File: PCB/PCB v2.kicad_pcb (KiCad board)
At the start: 4 copper layers, 55.3 x 42.7 mm, 91 parts, among them J1 Conn_01x02_Pin, J3 6871XX182122_687110182122, J5 Conn_01x03_Pin, J7 Conn_01x07_Pin, U1 LT3483AxS6, U11 OPA4350EA_250, U12 OPA4350EA_250, U13 OPA4350EA_250, U2 LT1761-2.5, U3 LT1964-BYP, U5 AD7606, U6 OPA4350EA_250

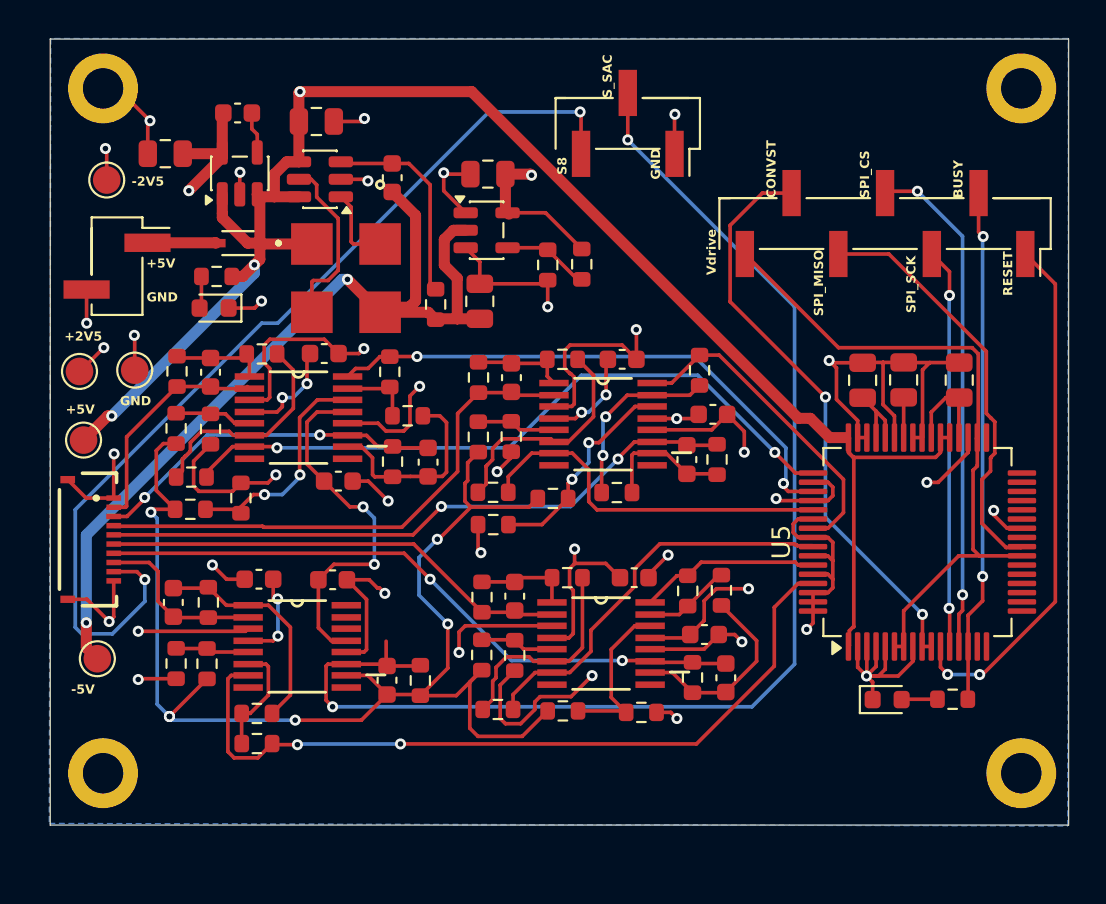
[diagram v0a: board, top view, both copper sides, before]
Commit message: Modifiche accordate fatte
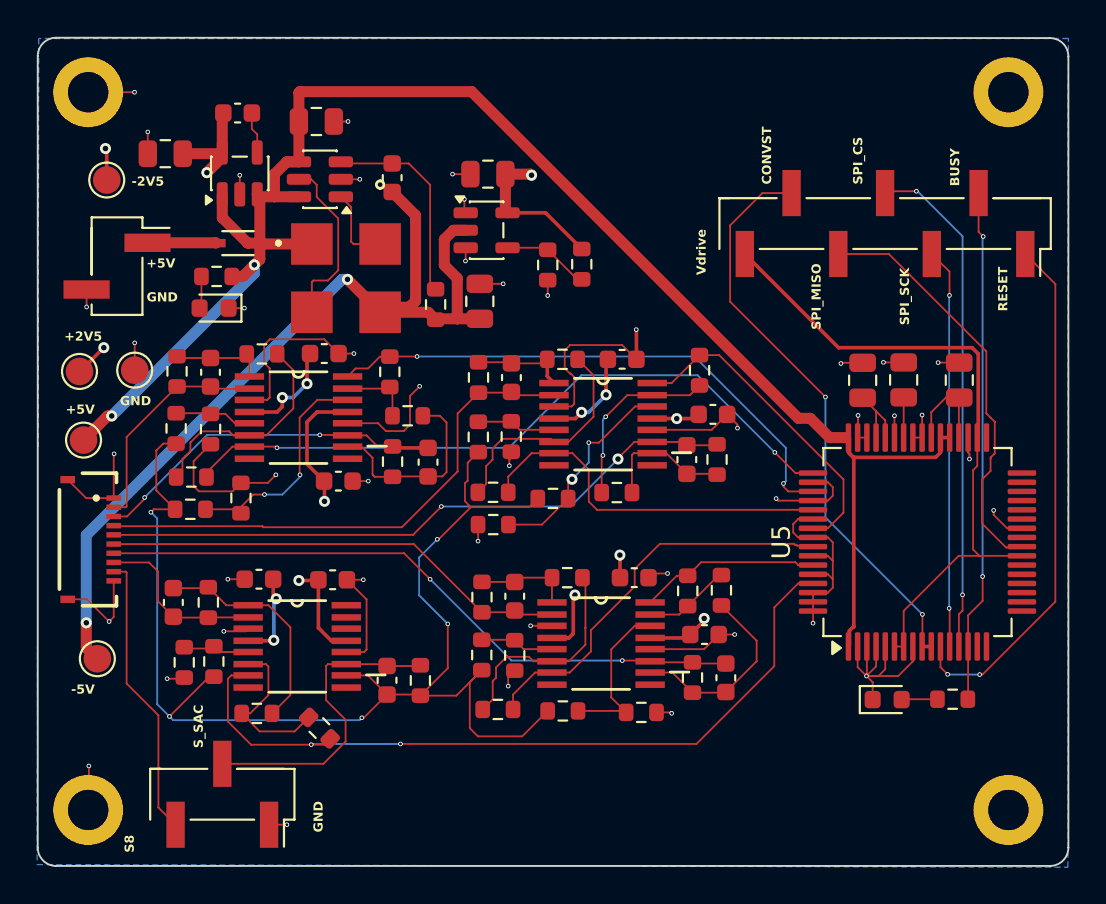
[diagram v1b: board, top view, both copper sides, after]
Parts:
- moved J5 42.6 mm to (131.3, 117.1)
- moved R59 3.50 mm to (136.6, 113.5), turned to -45 degrees
- moved H3 2.16 mm to (124.0, 118.0)
- moved H4 2.12 mm to (174.0, 118.0)
- moved H1 0.84 mm to (124.0, 79.0)
- moved H2 0.73 mm to (174.0, 79.0)
- moved R56 0.44 mm to (129.2, 110.0)
- moved R55 0.39 mm to (130.8, 109.9)
- turned R50 to 0 degrees
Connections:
- net BUSY renamed /POWER SUPPLY - ADC - SACRIFIED SENSOR/BUSY
- net CONVST renamed /POWER SUPPLY - ADC - SACRIFIED SENSOR/CONVST
- net RESET renamed /POWER SUPPLY - ADC - SACRIFIED SENSOR/RESET
- net SPI_CS renamed /POWER SUPPLY - ADC - SACRIFIED SENSOR/SPI_CS
- net SPI_MISO renamed /POWER SUPPLY - ADC - SACRIFIED SENSOR/SPI_MISO
- net SPI_SCK renamed /POWER SUPPLY - ADC - SACRIFIED SENSOR/SPI_SCK
- net V_sac renamed /SENSORS/V_sac
- net Vdrive renamed /POWER SUPPLY - ADC - SACRIFIED SENSOR/Vdrive
- net in-_b1 renamed /SENSORS/in-_b1
- net in-_b4 renamed /SENSORS/in-_b4
- net in-_c1 renamed /SENSORS/in-_c1
- net in-_c3 renamed /SENSORS/in-_c3
- net out_a1 renamed /SENSORS/out_a1
- net out_a4 renamed /SENSORS/out_a4
- net out_b1 renamed /SENSORS/out_b1
- net out_b3 renamed /SENSORS/out_b3
- C16 pad 1: out_a3 -> /SENSORS/out_a3
- R47 pad 1: out_a3 -> /SENSORS/out_a3
- R49 pad 1: in-_b3 -> /SENSORS/in-_b3
- R50 pad 1: in-_b3 -> /SENSORS/out_a3
- R50 pad 2: out_a3 -> /SENSORS/in-_b3
- U12 pad 1: out_a3 -> /SENSORS/out_a3
- U12 pad 6: in-_b3 -> /SENSORS/in-_b3
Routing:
- net GND: track 185.1 -> 128.4 mm, vias 35 -> 45
- net S_sac: track 69.8 -> 16.8 mm, vias 2 -> 0
- net S8: track 52.8 -> 15.5 mm, vias 2 -> 0
- net -2V5: track 40.3 -> 28.2 mm
- net in-_b3: track 11.7 -> 0.00 mm
- net /SENSORS/in-_b3: track 0.00 -> 11.6 mm
- net +2V5: track 34.2 -> 27.7 mm, vias 9 -> 10
- net out_a3: track 5.26 -> 0.00 mm
- net /SENSORS/out_a3: track 0.00 -> 4.91 mm
- net /SENSORS/in-_b4: track 6.21 -> 8.93 mm
- net /SENSORS/in-_b1: track 11.2 -> 12.1 mm
- net /SENSORS/out_b1: track 10.8 -> 10.1 mm
- net Net-(U1-FB): track 11.2 -> 10.5 mm
- net /SENSORS/out_a1: track 5.21 -> 4.54 mm
- net Net-(U6-+IN_D): track 12.5 -> 11.8 mm
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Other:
- board size 55.3 x 42.7 mm -> 56 x 45 mm
